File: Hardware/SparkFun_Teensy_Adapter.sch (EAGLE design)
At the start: 17 parts, among them J1 ARDUINO_R3_SHIELDUNO_R3_SHIEL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, J2 AVR_SPI_PRG_6PTH, U1 TEENSY-3.1

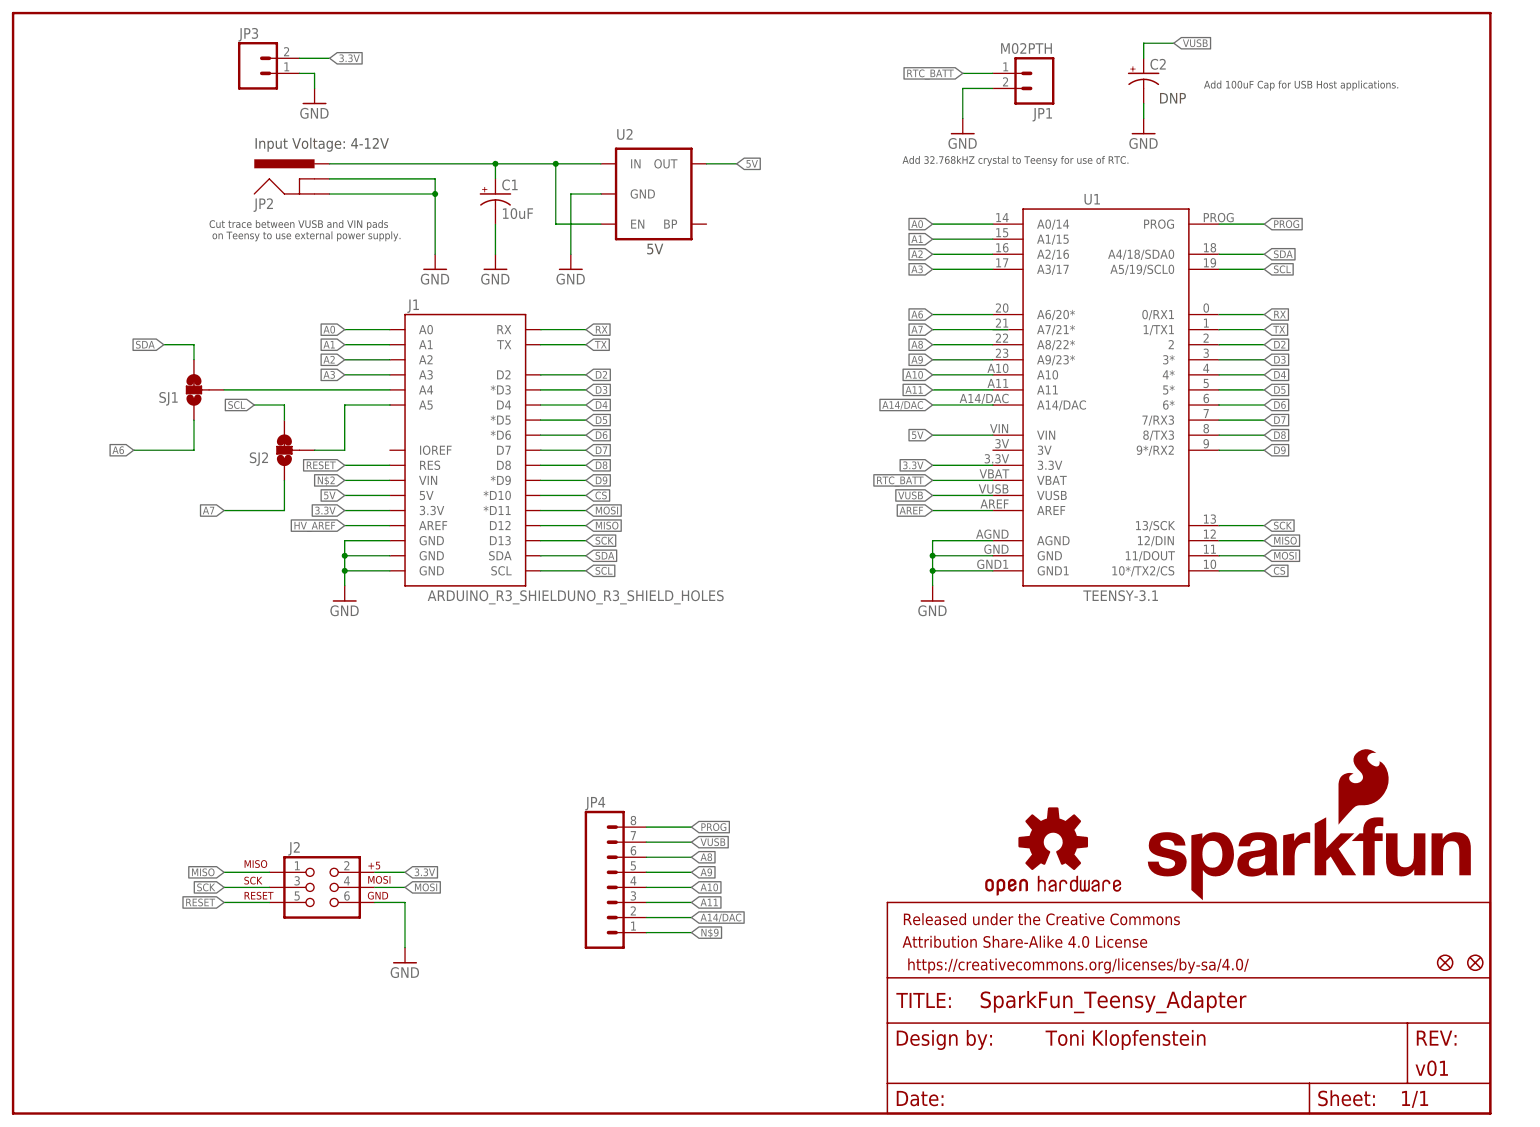
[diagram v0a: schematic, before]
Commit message: Routing finished
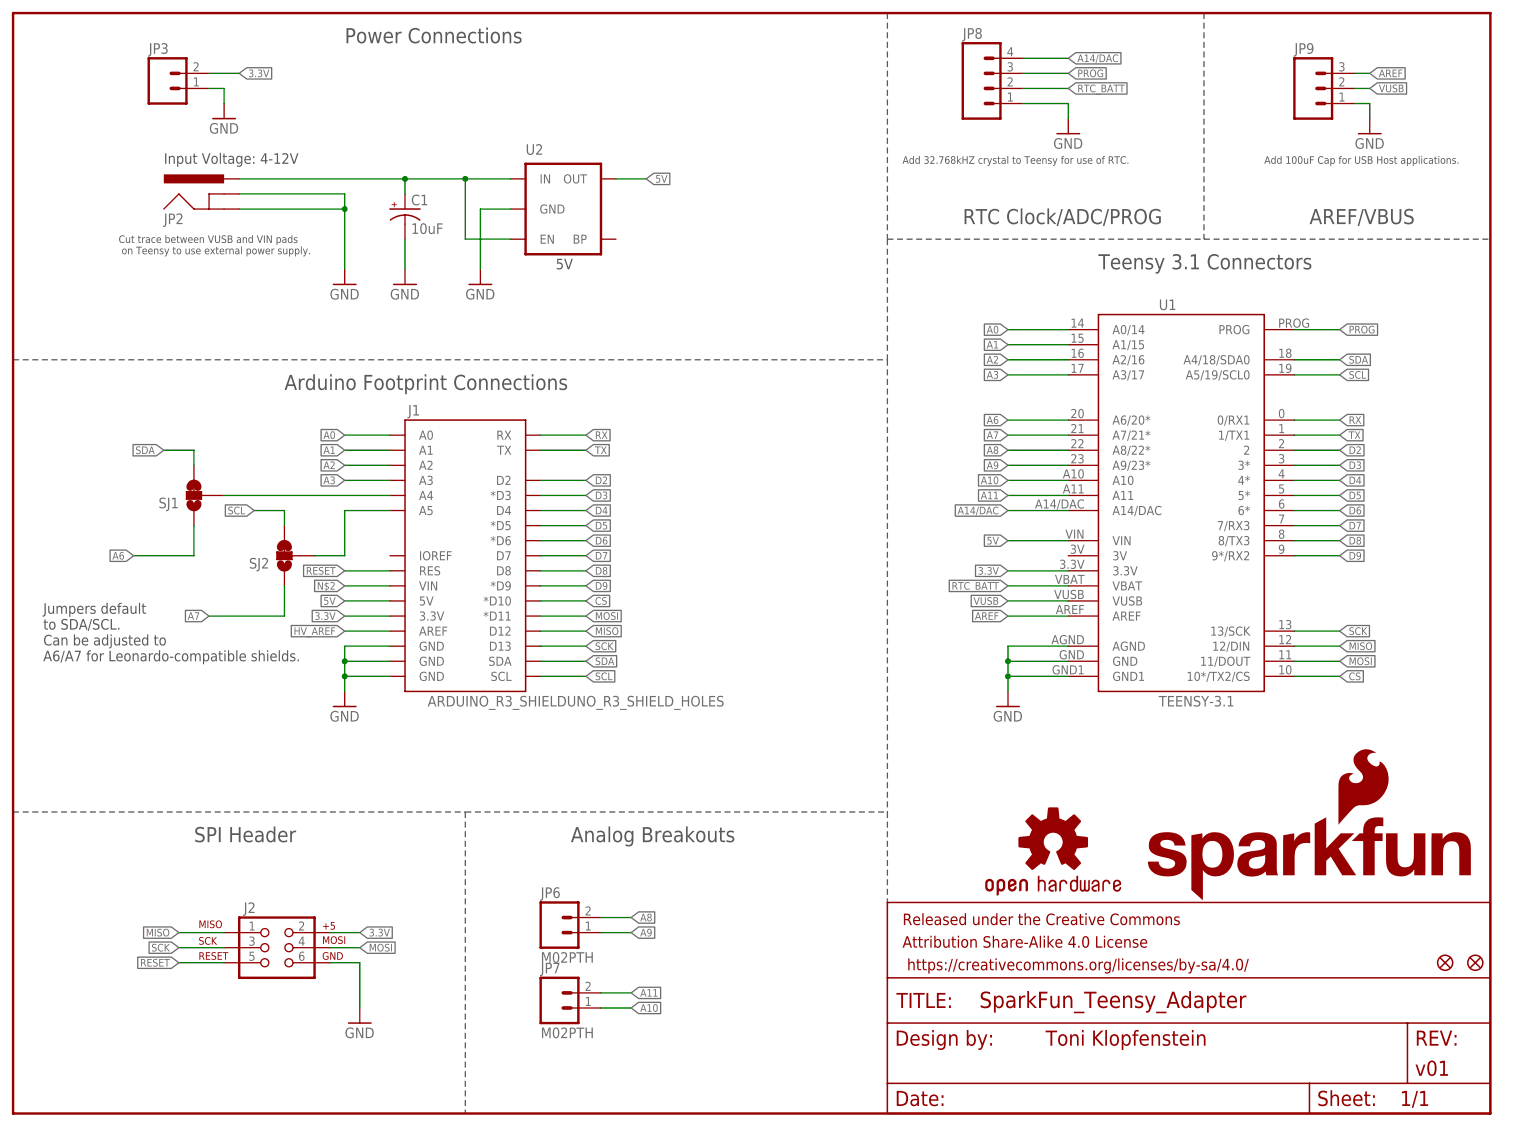
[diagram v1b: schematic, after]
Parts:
- removed C2: (no value), SparkFun-Capacitors:CAP_POL7343
- removed JP1: M02PTH, SparkFun-Connectors:M02PTH
- removed JP4: (no value), SparkFun-Connectors:M08
- added JP6, JP7: M02PTH, SparkFun-Connectors:M02PTH
- added JP8: (no value), SparkFun-Connectors:M04PTH
- added JP9: (no value), SparkFun-Connectors:M03PTH
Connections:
- removed net N$9: JP4.1
- net A10: now also JP7.1; no longer JP4.4
- net A11: now also JP7.2; no longer JP4.3
- net A14/DAC: now also JP8.4; no longer JP4.2
- net A7: now also U1.A7/21*
- net A8: now also JP6.2; no longer JP4.6
- net A9: now also JP6.1; no longer JP4.5
- net AREF: now also JP9.3
- net GND: now also JP8.1, JP9.1; no longer C2.-, JP1.2
- net PROG: now also JP8.3; no longer JP4.8
- net RTC_BATT: now also JP8.2; no longer JP1.1
- net VUSB: now also JP9.2; no longer C2.+, JP4.7
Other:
- note added: "AREF/VBUS"
- note added: "Analog Breakouts"
- note added: "Arduino Footprint Connections"
- note added: "Jumpers default to SDA/SCL. Can be adjusted to A6/A7 for Leonardo-compatible shields."
- note added: "Power Connections"
- note added: "RTC Clock/ADC/PROG"
- note added: "SPI Header"
- note added: "Teensy 3.1 Connectors"
- note removed: "DNP"
- moved on the sheet: C1, J1, J2, JP2, JP3, SJ1, SJ2, U1, U2
